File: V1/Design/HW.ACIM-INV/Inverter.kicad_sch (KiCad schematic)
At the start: 67 parts, among them J16 HIGH VOLTAGE OUTPUTS, J2 U, J3 V, J4 W, J5 N, J6 U, J7 V, J8 W, J9 N, M5 560V/1.75kA, M6 560V/1.75kA, M7 560V/1.75kA, Q3 20V/1A, U10 DIGI ISO, U11 I=±10A, U12 I=±10A, U13 CMP-1CH, U7 IPM 600V/15A, U8 DIGI ISO, U9 DIGI ISO

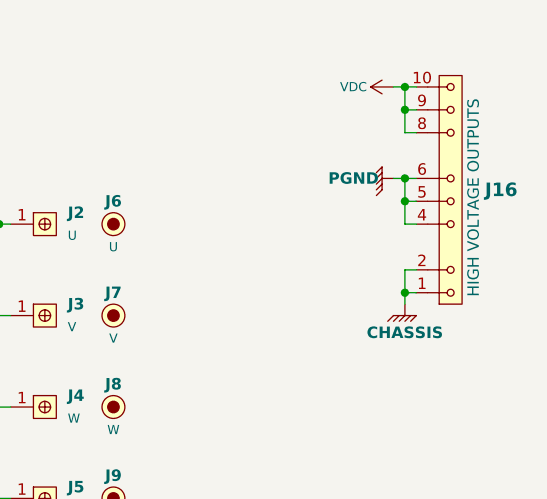
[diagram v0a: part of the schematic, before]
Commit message: V1 schematic update 20
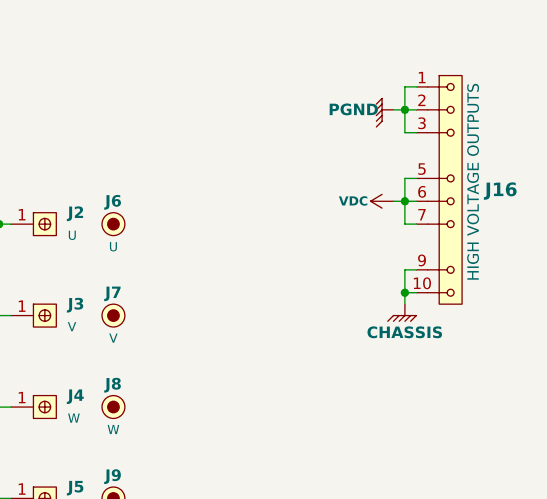
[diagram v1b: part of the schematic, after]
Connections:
- net CHASSIS: now also J16.10, J16.9; no longer J16.1, J16.2
- net PGND: now also J16.1, J16.2, J16.3; no longer J16.4, J16.5, J16.6
- net VDC: now also J16.5, J16.6, J16.7; no longer J16.10, J16.8, J16.9
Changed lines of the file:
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@@
 	)
 	(junction
-		(at 268.605 21.59)
-		(diameter 0)
-		(color 0 0 0 0)
-	)
-	(junction
 		(at 245.11 131.445)
 		(diameter 0)
@@
 	)
 	(junction
-		(at 268.605 31.75)
-		(diameter 0)
-		(color 0 0 0 0)
-	)
-	(junction
 		(at 202.565 46.99)
 		(diameter 0)
@@
 	(wire
 		(pts
-			(xy 267.335 31.75) (xy 268.605 31.75)
-		)
-		(stroke
-			(width 0.3)
-			(type default)
-		)
-	)
-	(wire
-		(pts
 			(xy 219.075 66.04) (xy 219.075 67.31)
 		)
@@
 	(wire
 		(pts
-			(xy 267.335 21.59) (xy 268.605 21.59)
-		)
-		(stroke
-			(width 0.3)
-			(type default)
-		)
-	)
-	(wire
-		(pts
 			(xy 207.01 57.15) (xy 219.075 57.15)
 		)
@@
 	(wire
 		(pts
+			(xy 267.335 34.29) (xy 268.605 34.29)
+		)
+		(stroke
+			(width 0.3)
+			(type default)
+		)
+	)
+	(wire
+		(pts
 			(xy 81.28 145.415) (xy 74.93 145.415)
 		)
@@
 	(wire
 		(pts
+			(xy 267.335 24.13) (xy 268.605 24.13)
+		)
+		(stroke
+			(width 0.3)
+			(type default)
+		)
+	)
+	(wire
+		(pts
 			(xy 40.005 34.29) (xy 40.005 35.56)
 		)
@@
 	(symbol
 		(lib_id "SAMPI:SIL10")
-		(at 269.875 48.26 0)
-		(mirror x)
+		(at 269.875 17.78 0)
 		(unit 1)
 		(exclude_from_sim no)
@@
 		)
 		(property "Value" "HIGH VOLTAGE OUTPUTS"
-			(at 276.225 22.86 90)
+			(at 276.225 43.18 90)
 			(effects
 				(font
@@
 		)
 		(property "Footprint" "SAMPI:HDF1x10x2.54_TH_RA"
-			(at 269.875 48.26 0)
+			(at 269.875 17.78 0)
 			(effects
 				(font
@@
 		)
 		(property "Datasheet" ""
-			(at 269.875 48.26 0)
+			(at 269.875 17.78 0)
 			(effects
 				(font
@@
 		)
 		(property "Description" "CONN HDR 10POS 0.1 TIN PCB R/A"
-			(at 269.875 48.26 0)
+			(at 269.875 17.78 0)
 			(effects
 				(font
@@
 		)
 		(property "MFT" "Sullins"
-			(at 269.875 48.26 0)
+			(at 269.875 17.78 0)
 			(effects
 				(font
@@
 		)
 		(property "MNP" "PPTC101LGBN-RC"
-			(at 269.875 48.26 0)
+			(at 269.875 17.78 0)
 			(effects
 				(font
@@
 		)
 		(property "Checked" "OK"
-			(at 269.875 48.26 0)
+			(at 269.875 17.78 0)
 			(effects
 				(font
@@
 		(pin "6"
 		)
-		(pin "8"
-		)
 		(pin "1"
 		)
@@
 		(pin "10"
 		)
-		(pin "4"
-		)
 		(pin "9"
 		)
 		(pin "5"
 		)
+		(pin "3"
+		)
+		(pin "7"
+		)
 		(instances
 			(project "HW.ACIM-INV"
@@
 	(symbol
 		(lib_id "power:VDC")
-		(at 267.335 21.59 90)
+		(at 267.335 34.29 90)
 		(unit 1)
 		(exclude_from_sim no)
@@
 		(dnp no)
 		(property "Reference" "#PWR0209"
-			(at 269.875 21.59 0)
+			(at 269.875 34.29 0)
 			(effects
 				(font
@@
 		)
 		(property "Value" "VDC"
-			(at 262.89 21.59 90)
+			(at 262.89 34.29 90)
 			(effects
 				(font
@@
 					(size 1.016 1.016)
 					(thickness 0.127)
+					(bold yes)
 				)
 			)
 		)
 		(property "Footprint" ""
-			(at 267.335 21.59 0)
+			(at 267.335 34.29 0)
 			(effects
 				(font
@@
 		)
 		(property "Datasheet" ""
-			(at 267.335 21.59 0)
+			(at 267.335 34.29 0)
 			(effects
 				(font
@@
 		)
 		(property "Description" ""
-			(at 267.335 21.59 0)
+			(at 267.335 34.29 0)
 			(effects
 				(font
@@
 	(symbol
 		(lib_id "SAMPI:PGND")
-		(at 267.335 31.75 270)
+		(at 267.335 24.13 270)
 		(mirror x)
 		(unit 1)
@@
 		(dnp no)
 		(property "Reference" "#PWR0207"
-			(at 262.255 31.75 0)
+			(at 262.255 24.13 0)
 			(effects
 				(font
@@
 		)
 		(property "Value" "PGND"
-			(at 262.89 31.75 90)
+			(at 262.89 24.13 90)
 			(effects
 				(font
@@
 		)
 		(property "Footprint" ""
-			(at 267.335 31.75 0)
+			(at 267.335 24.13 0)
 			(effects
 				(font
@@
 		)
 		(property "Datasheet" ""
-			(at 267.335 31.75 0)
+			(at 267.335 24.13 0)
 			(effects
 				(font
@@
 		)
 		(property "Description" ""
-			(at 267.335 31.75 0)
+			(at 267.335 24.13 0)
 			(effects
 				(font

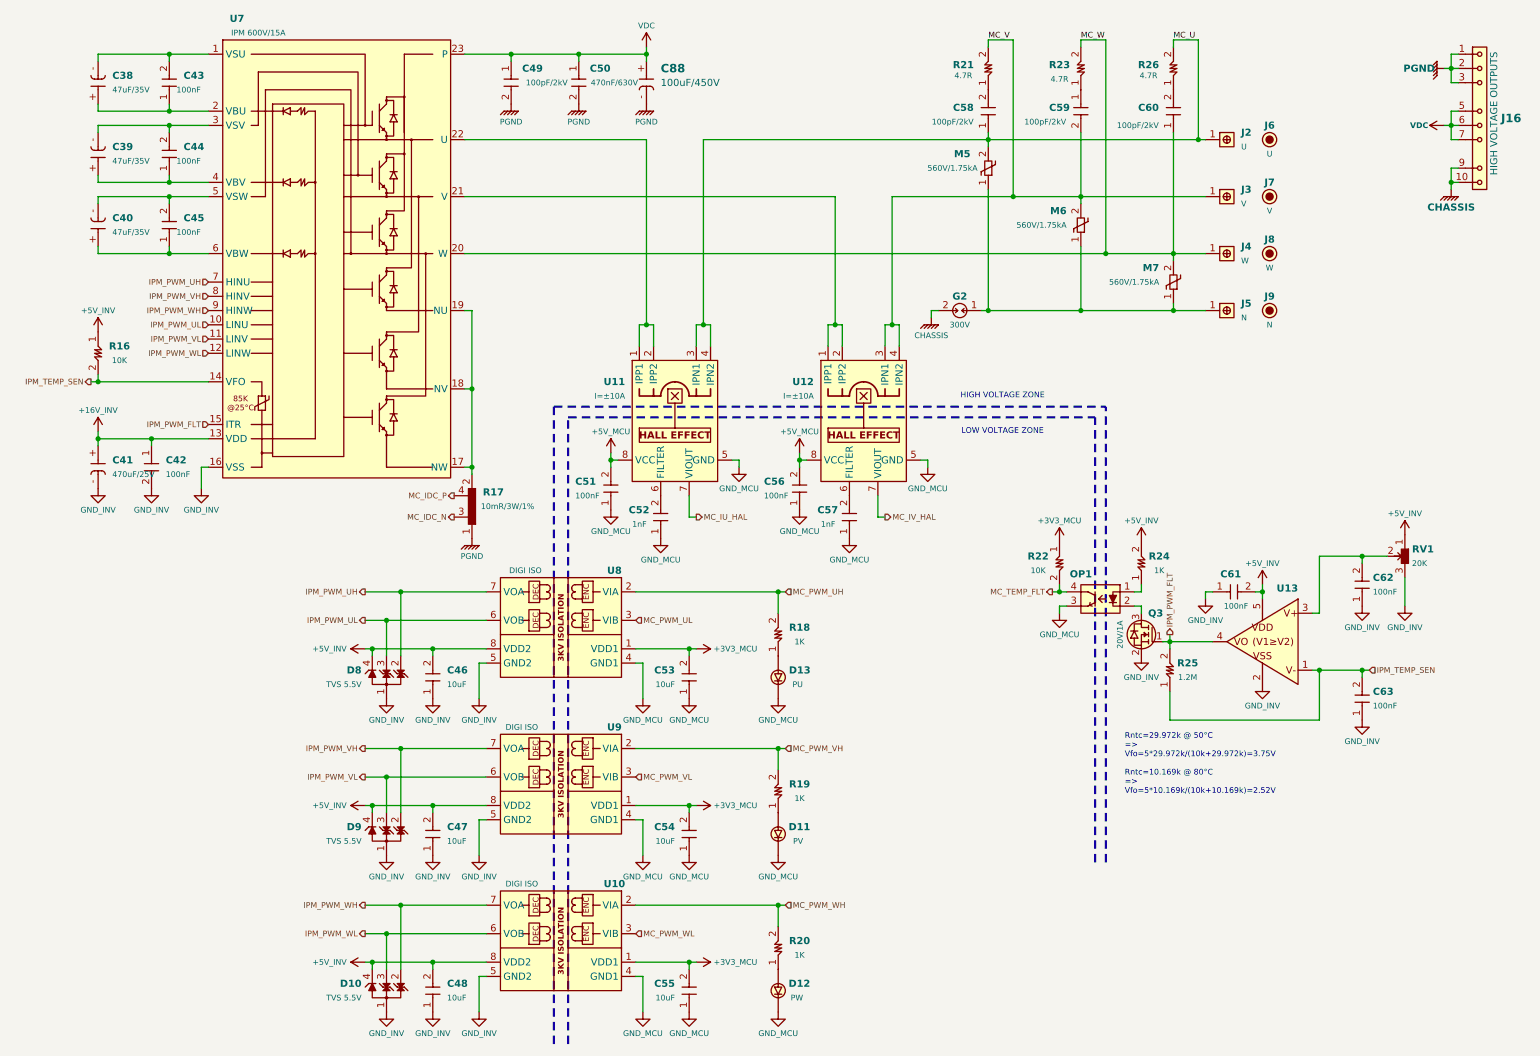
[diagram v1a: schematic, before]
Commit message: V1 schematic update 22
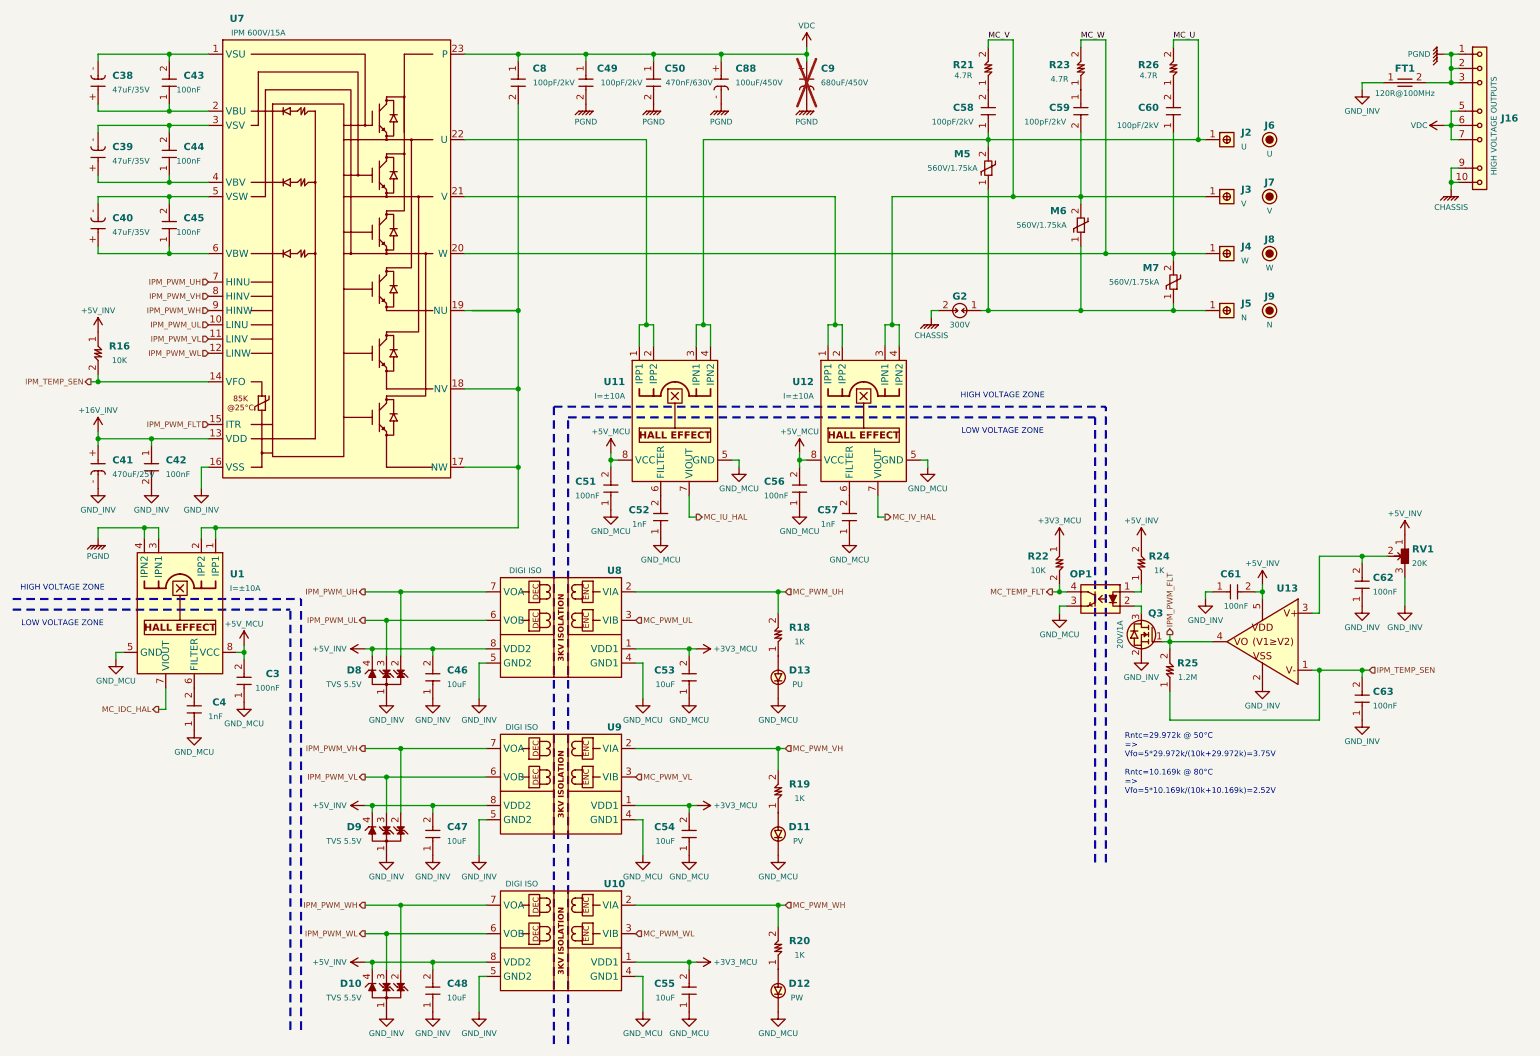
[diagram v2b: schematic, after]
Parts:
- removed R17: 10mR/3W/1%, SAMPI:SHU2512, symbol SAMPI:SHUNT
- added C3: 100nF, SAMPI:CAP0603, symbol SAMPI:CERCAP
- added C4: 1nF, SAMPI:CAP0603, symbol SAMPI:CERCAP
- added C8: 100pF/2kV, SAMPI:CAP1206, symbol SAMPI:CERCAP
- added C9: 680uF/450V, SAMPI:ESMQ451VSN681MA50S, symbol SAMPI:ELECCAP
- added FT1: 120R@100MHz, SAMPI:FT0603, symbol SAMPI:FerriteBead
- added U1: I=±10A, SAMPI:SOIC8_ALL, symbol SAMPI:ACS724
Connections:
- net +5V_MCU: now also C3.2, U1.8 (VCC)
- net GND_INV: now also FT1.1
- net GND_MCU: now also C3.1, C4.1, U1.5 (GND)
- net PGND: now also C9.-, FT1.2, U1.3 (IPN1), U1.4 (IPN2)
- net VDC: now also C8.1, C9.+
- net at U7.17 (NW), U7.18 (NV), U7.19 (NU): now also C8.2, U1.1 (IPP1), U1.2 (IPP2)
- new net: C4.2, U1.6 (FILTER)
- new net MC_IDC_HAL: U1.7 (VIOUT)
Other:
- moved on the sheet: C49, C50, C88
